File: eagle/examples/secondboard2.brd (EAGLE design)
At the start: 16.5 x 25.1 mm, 3 parts

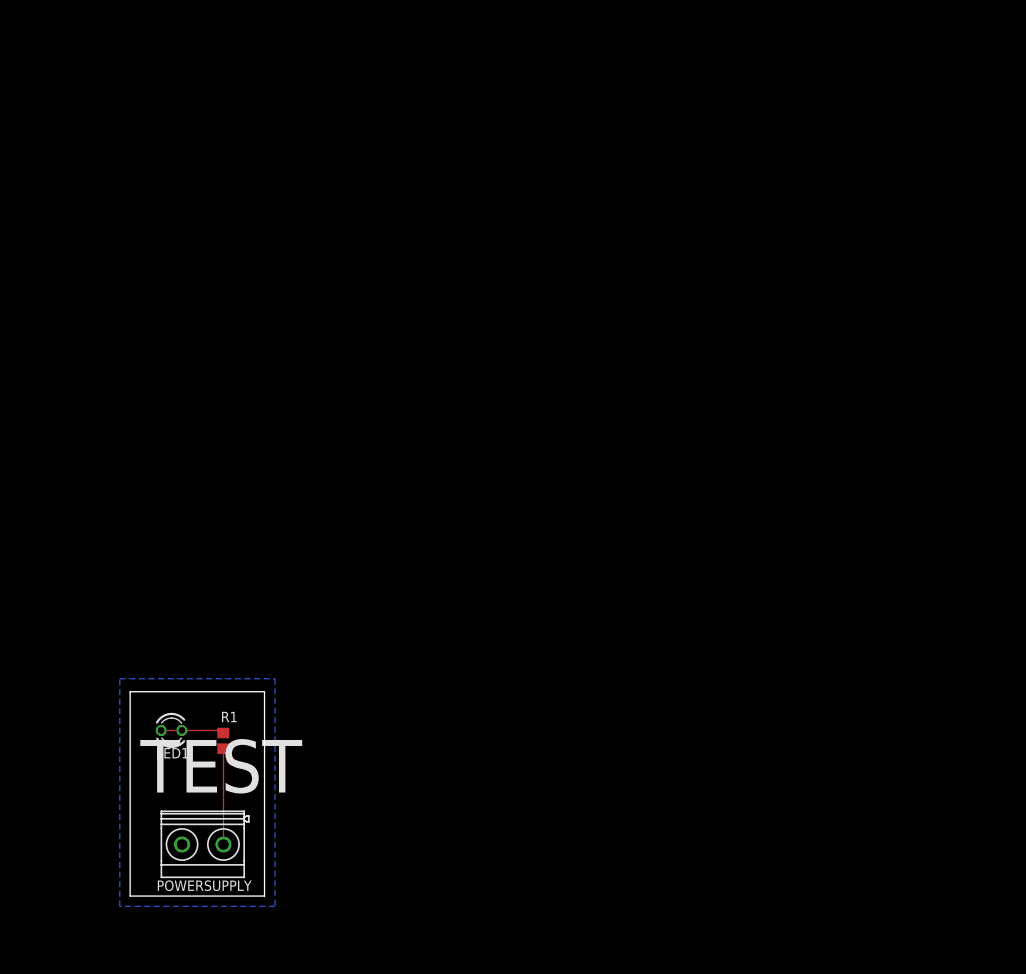
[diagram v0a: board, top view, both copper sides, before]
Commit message: examples
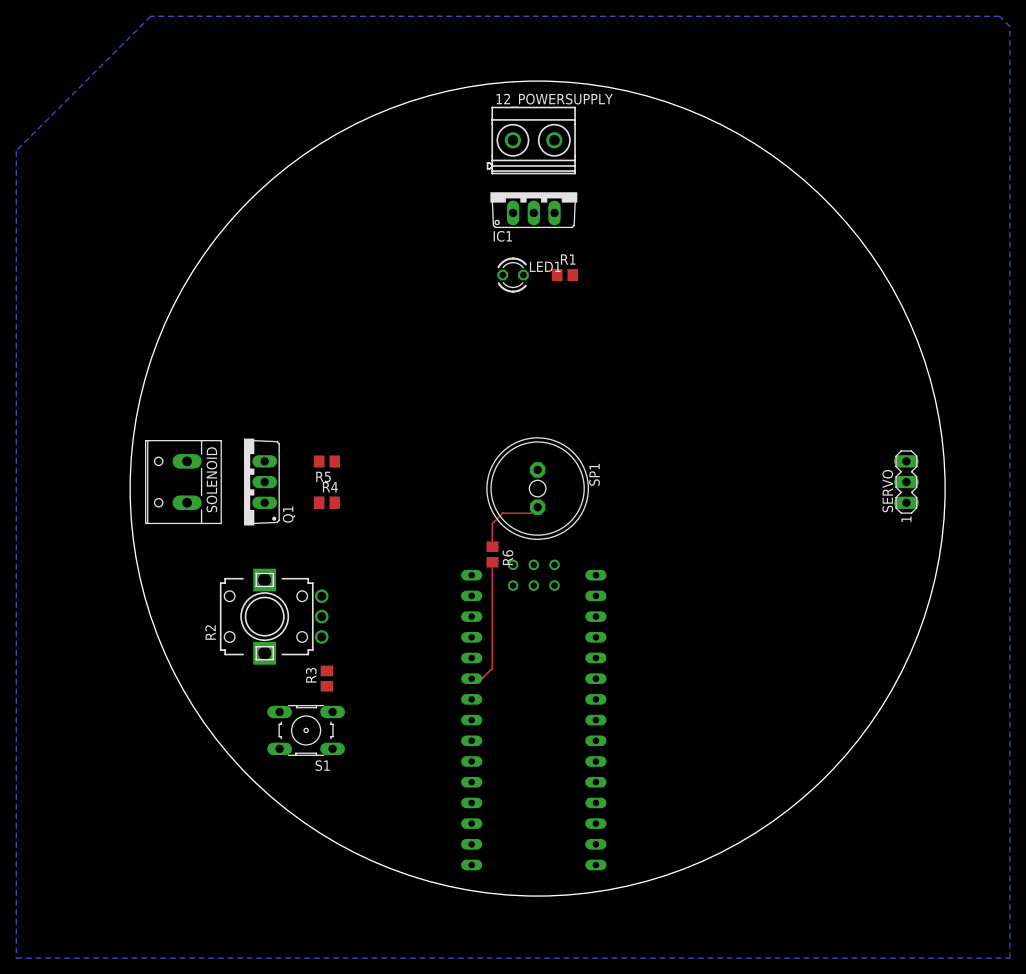
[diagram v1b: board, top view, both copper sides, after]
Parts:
- removed POWERSUPPLY: MKDSN1,5/2-5,08, con-phoenix-508:MKDSN1,5/2-5,08
- added 12_POWERSUPPLY: MKDSN1,5/2-5,08, con-phoenix-508:MKDSN1,5/2-5,08
- added IC1: 7805TV, linear:TO220V
- added Q1: IRF540, transistor-power:TO220BV
- added R2: EVUF3A, pot:EVUF
- added R3: 10K, rcl:R0805
- added R4: 1K, rcl:R0805
- added R5: 100K, rcl:R0805
- added R6: 100, rcl:R0805
- added S1: (no value), switch-omron:B3F-10XX
- added SERVO: (no value), con-lstb:MA03-1
- added SOLENOID: (no value), con-wago-508:W237-132
- added SP1: AL11P, buzzer:AL11P
- added U$1: NANO, Arduino-clone:NANO
- moved R1 70.9 mm to (53.3, 76.2), turned to 0 degrees
- moved LED1 69.9 mm to (47.0, 76.2)
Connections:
- new net +12V: 12_POWERSUPPLY.1, IC1.1, SOLENOID.2
- new net BUTTON: S1.4, U$1.D2
- new net BUZZ: R6.2, U$1.D3
- new net MOSFET: R4.2, U$1.D12
- new net N$1: R3.1, S1.3
- new net N$2: R6.1, SP1.+
- new net N$3: Q1.D, SOLENOID.1
- new net N$4: SERVO.3, U$1.D6
- new net N$6: Q1.G, R4.1, R5.1
- new net POT_OUT: R2.2, U$1.A0
- net +5V: now also IC1.3, R2.3, S1.1, SERVO.2, U$1.5V; no longer POWERSUPPLY.1
- net GND: now also 12_POWERSUPPLY.2, IC1.2, Q1.S, R2.1, R3.2, R5.2, SERVO.1, SP1.-, U$1.GND; no longer POWERSUPPLY.2
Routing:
- net BUZZ: track 0.00 -> 16.1 mm
- net +5V: track 11.8 -> 0.00 mm
- net N$2: track 0.00 -> 9.24 mm
- net CONNECT: track 7.75 -> 0.00 mm
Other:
- board size 16.5 x 25.1 mm -> 100 x 100 mm
- board text removed: "TEST"
